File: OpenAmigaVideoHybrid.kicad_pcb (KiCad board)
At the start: 2 copper layers, 56.4 x 21.5 mm, 59 parts, among them J1 CONN_MAINBOARD, J2 SVIDEO_OUT, Q1 2N3904, Q2 2N3904, Q3 2N3904, Q4 2N3904, U2 AD724, Y2 4.433619M

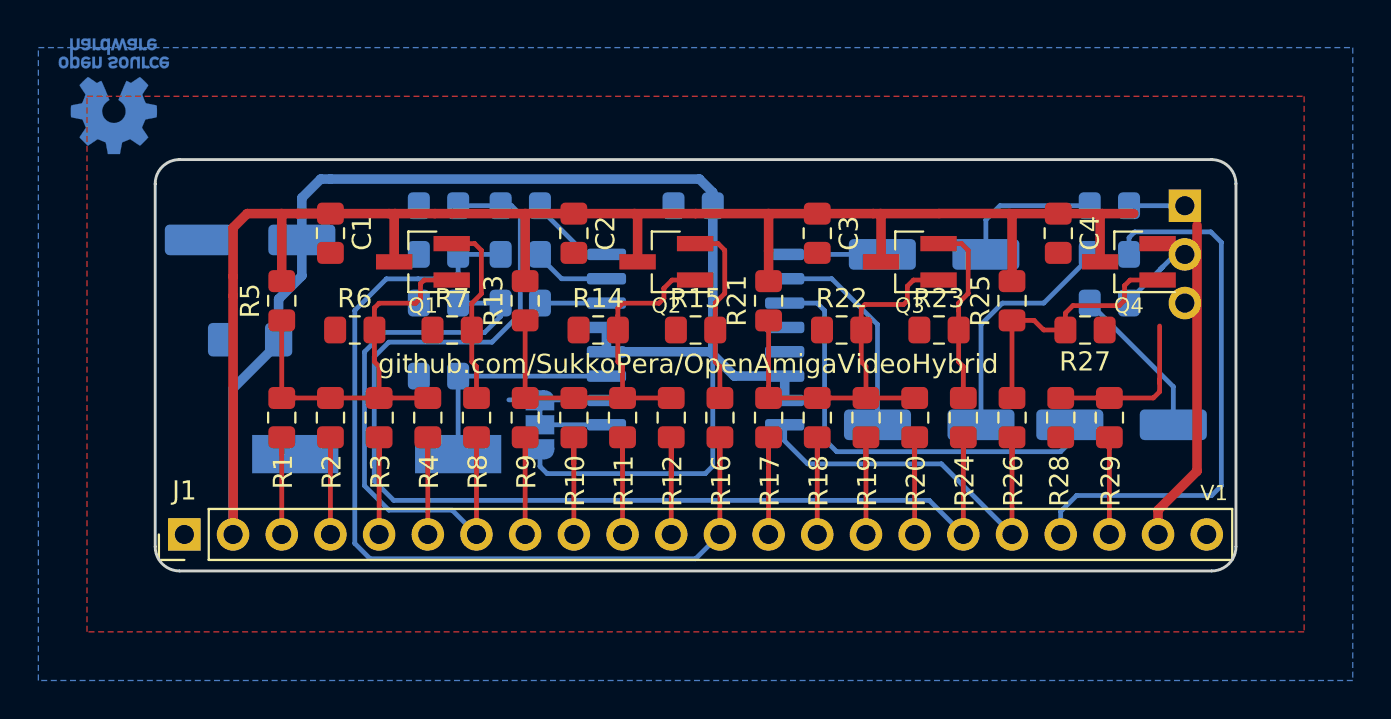
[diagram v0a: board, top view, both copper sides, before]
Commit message: THERE! Just needs some polishing!
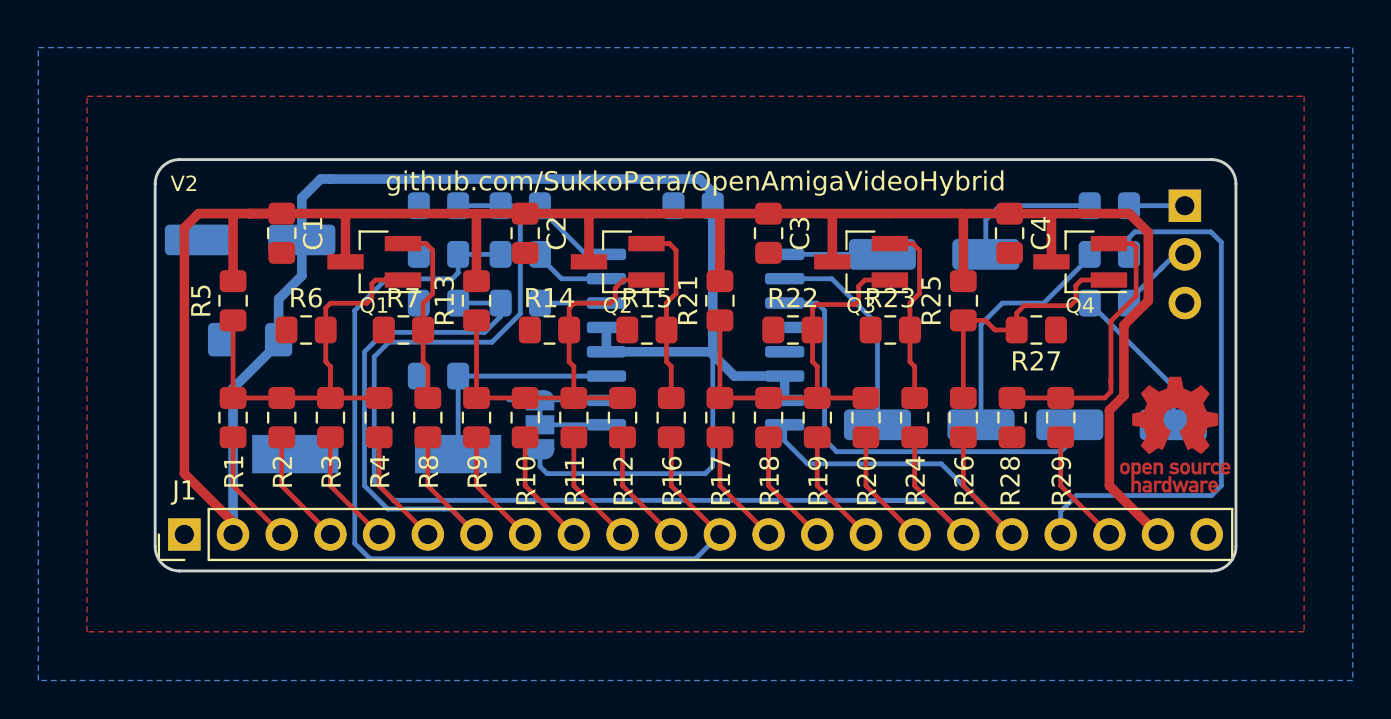
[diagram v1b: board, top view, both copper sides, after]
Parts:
- V0: moved to F.Cu
- moved V0 58.1 mm to (171.1, 119.3)
- moved C4 2.54 mm to (162.4, 108.7)
- moved Q2 2.54 mm to (142.0, 110.2)
- moved R11 2.54 mm to (139.7, 118.4)
- moved R15 2.54 mm to (143.5, 113.8)
- moved R17 2.54 mm to (147.3, 118.4)
- moved R21 2.54 mm to (147.3, 112.3)
- moved R24 2.54 mm to (157.5, 118.4)
- moved R4 2.54 mm to (129.5, 118.4)
- moved C1 2.54 mm to (124.5, 108.7)
- moved R2 2.54 mm to (124.5, 118.4)
- moved R6 2.54 mm to (125.7, 113.8)
- moved C2 2.54 mm to (137.2, 108.7)
- moved C3 2.54 mm to (149.9, 108.7)
- moved Q1 2.54 mm to (129.3, 110.2)
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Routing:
- net Net-(Q4-Pad1): track 8.88 -> 15.0 mm
- net VAA: track 184.2 -> 189.6 mm
- net /blue: track 61.5 -> 64.5 mm
- net /sync: track 4.61 -> 6.12 mm
- net /db0: track 6.96 -> 6.12 mm
- net /dr3: track 5.37 -> 6.12 mm
- net /dr2: track 5.50 -> 6.12 mm
- net /dr1: track 5.50 -> 6.12 mm
- net /db2: track 5.50 -> 6.12 mm
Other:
- board text added: "V2"
- board text removed: "V1"
